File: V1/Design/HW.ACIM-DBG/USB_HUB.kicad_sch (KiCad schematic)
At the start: 60 parts, among them J4 USB, U2 USB HUB 2.0 4-CH, U4 24MHz (3225), U9 USB HUB

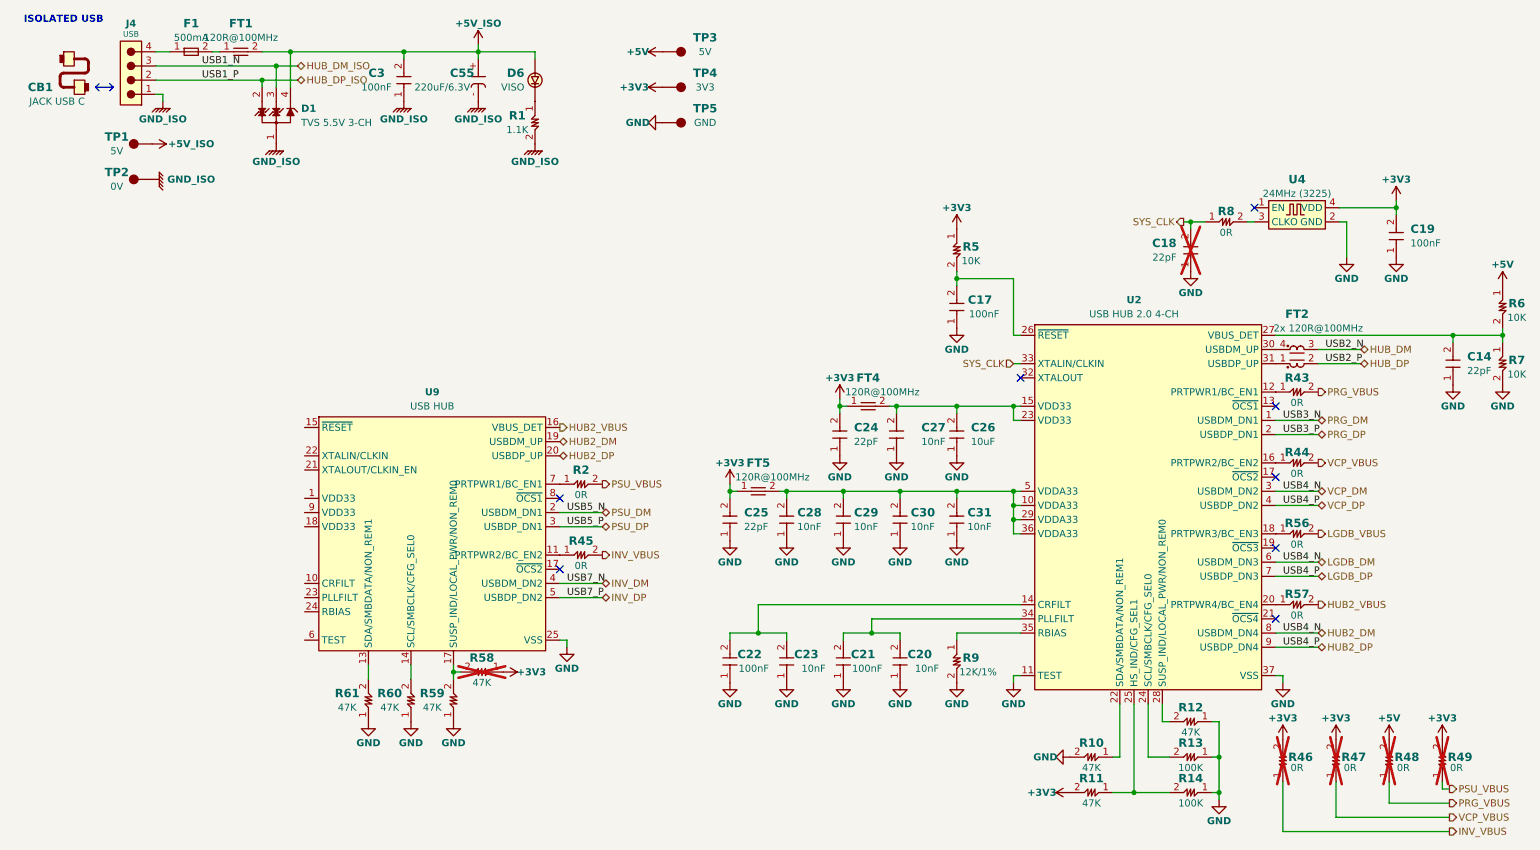
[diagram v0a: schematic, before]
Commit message: V1 schematic update 1
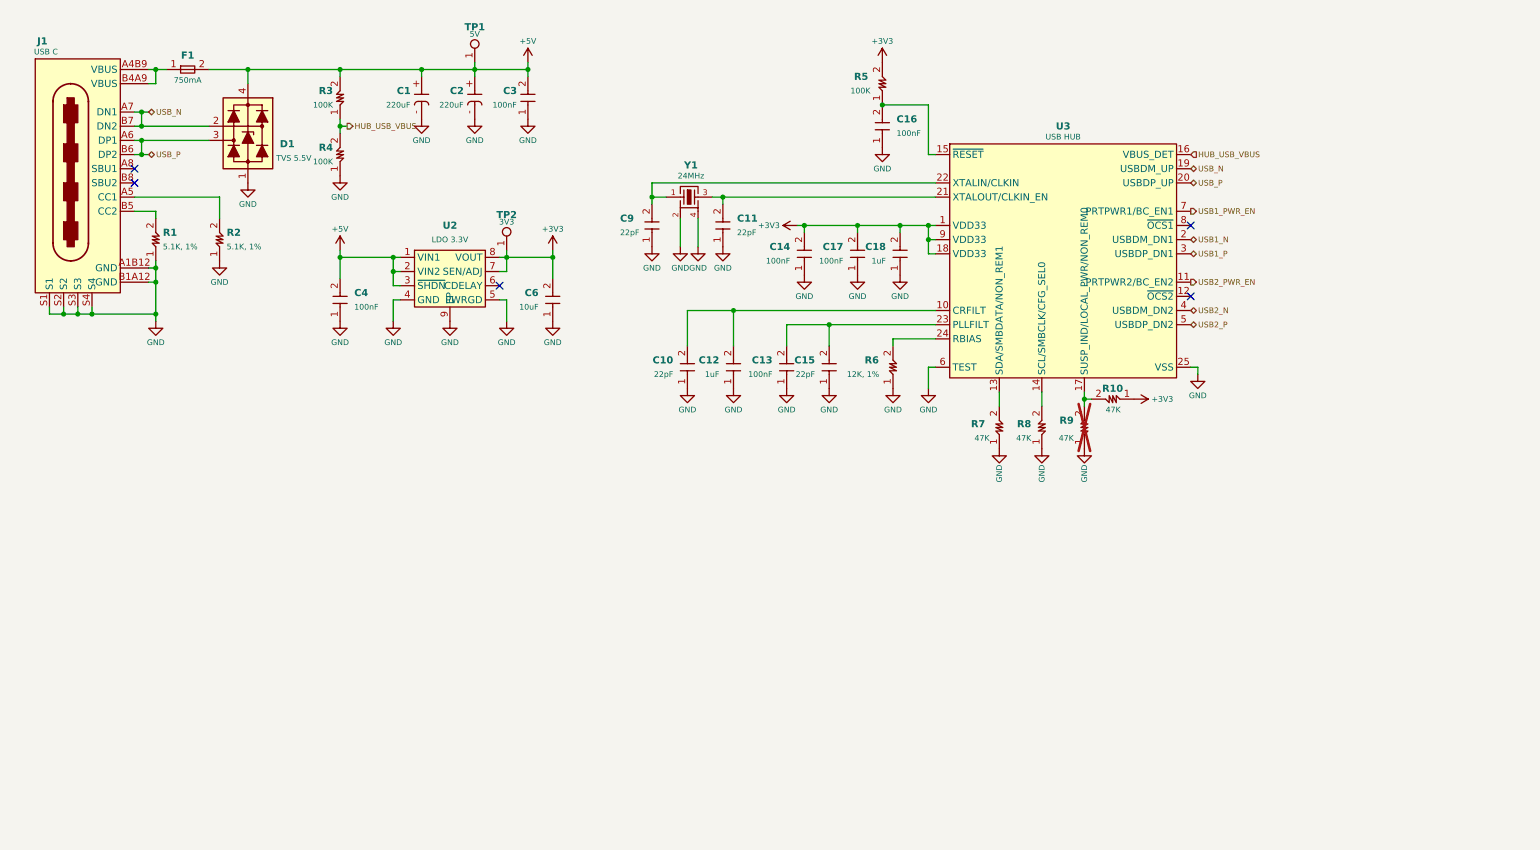
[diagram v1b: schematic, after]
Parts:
- removed C19, C21, C22: 100nF, SAMPI:CAP0603, symbol SAMPI:CERCAP
- removed C20, C23, C27, C28, C29, C30, C31: 10nF, SAMPI:CAP0603, symbol SAMPI:CERCAP
- removed C24, C25: 22pF, SAMPI:CAP0603, symbol SAMPI:CERCAP
- removed C26: 10uF, SAMPI:CAP0603, symbol SAMPI:CERCAP
- removed C55: 220uF/6.3V, SAMPI:CAP1411, symbol SAMPI:ELECCAP
- removed CB1: JACK USB C, symbol SAMPI:CABLE1
- removed D1: TVS 5.5V 3-CH, SAMPI:SOT143B_NEXT, symbol SAM1:TVS_3CH
- removed D6: VISO, SAMPI:LED0603, symbol SAMPI:WLED
- removed F1: 500mA, SAMPI:FUSE0805, symbol SAM1:FUSE
- removed FT1: 120R@100MHz, SAMPI:FT0603, symbol SAM1:FerriteBead
- removed FT2: 2x 120R@100MHz, SAMPI:IND1210_4P, symbol SAMPI:IND1210_4P
- removed FT4, FT5: 120R@100MHz, SAMPI:FT0603, symbol SAMPI:FerriteBead
- removed J4: USB, SAMPI:HDM-1x4x2.54-TH-RA, symbol SAMPI:SIL04-1
- removed R11, R12, R58, R59, R60, R61: 47K, SAMPI:RES0603, symbol SAMPI:RES
- removed R13, R14: 100K, SAMPI:RES0603, symbol SAMPI:RES
- removed R43, R44, R45, R46, R47, R48, R49, R56, R57: 0R, SAMPI:RES0603, symbol SAMPI:RES
- removed TP1, TP3: 5V, SAMPI:TP1MM, symbol SAMPI:TESTPOINT
- removed TP2: 0V, SAMPI:TP1MM, symbol SAMPI:TESTPOINT
- removed TP4: 3V3, SAMPI:TP1MM, symbol SAMPI:TESTPOINT
- removed TP5: GND, SAMPI:TP1MM, symbol SAMPI:TESTPOINT
- removed U2: USB HUB 2.0 4-CH, SAMPI:SQFN36_6x6_MCHP, symbol SAMPI:USB2514B
- removed U4: 24MHz (3225), SAMPI:CDFN3225-4LD-PL-1, symbol SAMPI:OSC
- removed U9: USB HUB, symbol SAMPI:USB2422
- added C1, C2: 220uF, Liem:CAP2312-6032, symbol SAMPI:ELECCAP
- added C10, C11, C15, C9: 22pF, Liem:CAP0402, symbol SAMPI:CERCAP
- added C12: 1uF, Liem:CAP0402, symbol SAMPI:CERCAP
- added C13, C16, C4: 100nF, Liem:CAP0402, symbol SAMPI:CERCAP
- added C6: 10uF, Liem:CAP0603, symbol SAMPI:CERCAP
- added D1: TVS 5.5V, Liem:SOT143B_NEXT, symbol Liem:PRTR5V0U2X
- added F1: 750mA, tuanlib:FUSE_ 1206, symbol Liem:FUSE
- added J1: USB C, Liem:USB4105, symbol Liem:USB4105
- added R3, R4: 100K, Liem:RES0402, symbol SAMPI:RES
- added TP1: 5V, tuanlib:TestPoint, symbol My_Library:TestPoint
- added TP2: 3V3, tuanlib:TestPoint, symbol My_Library:TestPoint
- added U2: LDO 3.3V, Liem:DFN8_3x3_MCHP, symbol Liem:MCP1727
- added U3: USB HUB, Package_DFN_QFN:QFN-24-1EP_4x4mm_P0.5mm_EP2.8x2.8mm, symbol SAMPI:USB2422
- added Y1: 24MHz, Liem:CDFN3225-4LD-PL-1, symbol TUANLIB:FA-20H
- C14: value 22pF -> 100nF; footprint SAMPI:CAP0603 -> Liem:CAP0402; Checked OK -> (none); MFT Walsin -> Walsin Technology Corporation; MNP 0603N220J500CT -> 0402B104K160CT; Unit Price 0.012 -> (none)
- C17, C3: footprint SAMPI:CAP0603 -> Liem:CAP0402; Checked OK -> (none); MFT Samsung -> Walsin Technology Corporation; MNP CL10B104KB8NNNC -> 0402B104K160CT; Unit Price 0.0146 -> (none)
- C18: value 22pF -> 1uF; footprint SAMPI:CAP0603 -> Liem:CAP0402; Checked OK -> (none); MFT Walsin -> Murata Electronics; MNP 0603N220J500CT -> GRM155R60J105KE19D; Unit Price 0.012 -> (none); now fitted; now in the parts list
- R1: value 1.1K -> 5.1K, 1%; footprint SAMPI:RES0603 -> Liem:RES0402; Checked OK -> (none); MNP AC0603FR-071K1L -> RC0402FR-075K1L; Unit Price 0.021 -> (none)
- R10: footprint SAMPI:RES0603 -> Liem:RES0402; Checked OK -> (none); MFT YAGEO -> Rohm Semiconductor; MNP RC0603FR-0747KL -> MCR01MZPJ473; Unit Price 0.019 -> (none)
- R2: value 0R -> 5.1K, 1%; footprint SAMPI:RES0603 -> Liem:RES0402; Checked OK -> (none); MNP RC0603JR-070RL -> RC0402FR-075K1L; Unit Price 0.015 -> (none)
- R5: value 10K -> 100K; footprint SAMPI:RES0603 -> Liem:RES0402; Checked OK -> (none); MFT YAGEO -> Rohm Semiconductor; MNP RC0603FR-0710KL -> MCR01MRTJ104; Unit Price 0.019 -> (none)
- R6: value 10K -> 12K, 1%; footprint SAMPI:RES0603 -> Liem:RES0402; Checked OK -> (none); MNP RC0603FR-0710KL -> RC0402FR-0712KL; Unit Price 0.019 -> (none)
- R7: value 10K -> 47K; footprint SAMPI:RES0603 -> Liem:RES0402; Checked OK -> (none); MFT YAGEO -> Rohm Semiconductor; MNP RC0603FR-0710KL -> MCR01MZPJ473; Unit Price 0.019 -> (none)
- R8: value 0R -> 47K; footprint SAMPI:RES0603 -> Liem:RES0402; Checked OK -> (none); MFT YAGEO -> Rohm Semiconductor; MNP RC0603JR-070RL -> MCR01MZPJ473; Unit Price 0.015 -> (none)
- R9: value 12K/1% -> 47K; footprint SAMPI:RES0603 -> Liem:RES0402; Checked OK -> (none); MFT YAGEO -> Rohm Semiconductor; MNP RC0603FR-0712KL -> MCR01MZPJ473; Unit Price 0.019 -> (none); now not fitted; now left out of the parts list
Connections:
- net +5V_ISO is gone; now on net +5V: C3.2
- net +3V3: now also C14.2, C17.2, C18.2, R10.1, R5.2, C6.2, TP2.1, U2.7 (SEN/ADJ), U2.8 (VOUT), U3.1 (VDD33), U3.18 (VDD33), U3.9 (VDD33); no longer R5.1
- net +5V: now also C1.+, C2.+, C4.2, D1.4 (VCC), F1.2, R3.2, TP1.1, U2.1 (VIN1), U2.2 (VIN2), U2.3 (~{SHDN}); no longer R6.1
- net GND: now also C3.1, R1.1, R2.1, R6.1, R7.1, R8.1, R9.1, C1.-, C10.1, C11.1, C12.1, C13.1, C15.1, C16.1, C2.-, C4.1, C6.1, C9.1, D1.1 (GND), J1.A1B12 (GND), J1.B1A12 (GND), J1.S1, J1.S2, J1.S3, J1.S4, R4.1, U2.4 (GND), U2.5 (PWRGD), U2.9 (EP), U3.25 (VSS), U3.6 (TEST), Y1.2, Y1.4; no longer R10.2, R7.2, R9.2
- net at R8.2: now also U3.14 (SCL/SMBCLK/CFG_SEL0)
- net GND_ISO: no longer names the net of R1.2
- net GND_ISO: now also J1.B5 (CC2); no longer C3.1
- net PSU_VBUS: no longer names the net of R2.2
- net PSU_VBUS: now also J1.A5 (CC1)
- removed net SYS_CLK: C18.2, R8.1
- new net: C9.2, U3.22 (XTALIN/CLKIN), Y1.1
- new net: C11.2, U3.21 (XTALOUT/CLKIN_EN), Y1.3
- new net: C16.2, R5.1, U3.15 (~{RESET})
- new net: R7.2, U3.13 (SDA/SMBDATA/NON_REM1)
- new net: C13.2, C15.2, U3.23 (PLLFILT)
- new net: F1.1, J1.A4B9 (VBUS), J1.B4A9 (VBUS)
- new net: R10.2, R9.2, U3.17 (SUSP_IND/LOCAL_PWR/NON_REM0)
- new net: C10.2, C12.2, U3.10 (CRFILT)
- new net: R6.2, U3.24 (RBIAS)
- new net HUB_USB_VBUS: R3.1, R4.2, U3.16 (VBUS_DET)
- new net USB1_N: U3.2 (USBDM_DN1)
- new net USB1_P: U3.3 (USBDP_DN1)
- new net USB1_PWR_EN: U3.7 (PRTPWR1/BC_EN1)
- new net USB2_N: U3.4 (USBDM_DN2)
- new net USB2_P: U3.5 (USBDP_DN2)
- new net USB2_PWR_EN: U3.11 (PRTPWR2/BC_EN2)
- new net USB_N: D1.2 (I/O1), J1.A7 (DN1), J1.B7 (DN2), U3.19 (USBDM_UP)
- new net USB_P: D1.3 (I/O2), J1.A6 (DP1), J1.B6 (DP2), U3.20 (USBDP_UP)
- no-connect marks 8 -> 5
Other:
- note removed: "ISOLATED USB"
